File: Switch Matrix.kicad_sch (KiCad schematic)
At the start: 131 parts, among them SW1 SD_6B1D, SW10 SD_4B1E, SW100 SD_4B3E, SW101 SD_4B3E, SW102 SD_4B3E, SW103 SD_4B3E, SW104 SD_4B3E, SW105 SD_4B3E, SW106 SD_4B3E, SW107 SD_4B3E, SW108 SD_4B3E, SW109 SD_4B3E, SW11 SD_4B1E, SW110 SD_4B3E, SW111 SD_4B3E, SW112 SD_6B1D, SW113 SD_4B3E, SW114 SD_4B3E, SW115 UNPOPULATED, SW116 SD_4B3E, SW117 SD_5B3E, SW118 SD_4B3E, SW119 UNPOPULATED, SW12 SD_6B1D, SW120 SD_4B3E, SW121 SD_4B3E, SW122 SD_4B3E, SW122a0 UNPOPULATED, SW123 SD_4B3E, SW123a0 UNPOPULATED, SW124 UNPOPULATED, SW124a0 SD_4B3E, SW125 SD_4B3E, SW126 SD_4B3E, SW127 UNPOPULATED, SW128 SD_4B3E, SW13 SD_4B1E, SW14 SD_6B1D, SW15 SD_4B1E, SW16 SD_6B1D, SW17 SD_4B1E, SW18 SD_6B1D, SW19 SD_4B1E, SW2 SD_4B1E, SW20 SD_6B1D, SW21 SD_4B1E, SW22 SD_6B1D, SW23 SD_4B1E, SW24 SD_6B1D, SW25 SD_4B3E, SW26 SD_4B3E, SW27 SD_6B1D, SW28 SD_4B3E, SW29 SD_4B3E, SW3 SD_6B1D, SW30 SD_4B3E, SW31 SD_4B3E, SW32 SD_4B3E, SW33 SD_4B3E, SW34 SD_4B3E, SW35 SD_4B3E, SW36 SD_4B3E, SW37 SD_4B3E, SW38 SD_4B3E, SW39 SD_4B3E, SW4 SD_4B1E, SW40 SD_4B3E, SW41 UNPOPULATED, SW42 SD_4B3E, SW43 SD_4B3E, SW44 SD_4B3E, SW45 SD_4B3E, SW46 SD_6B1D, SW47 SD_4B3E, SW48 SD_4B3E, SW49 SD_4B3E, SW5 SD_6B1D, SW50 SD_4B3E, SW51 SD_4B3E, SW52 SD_6B1D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

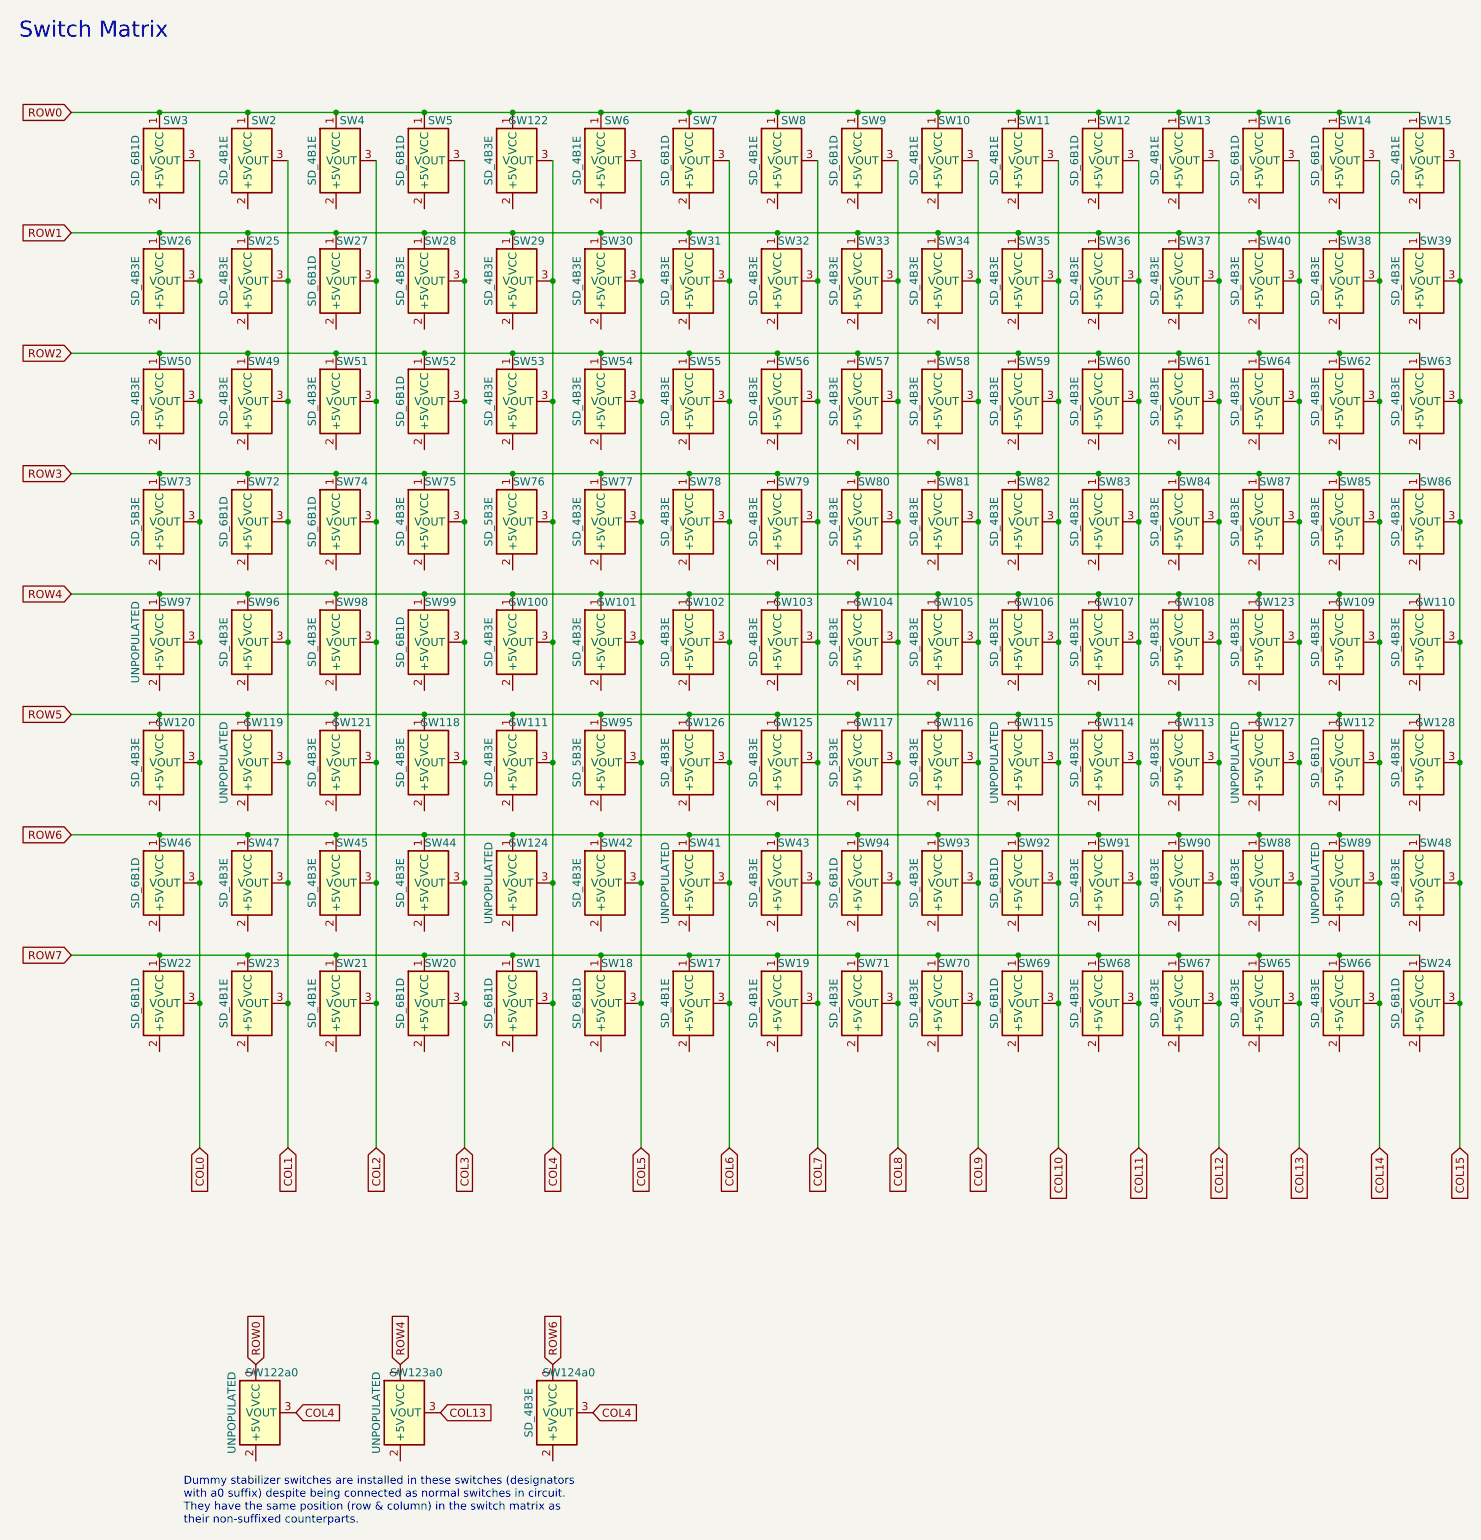
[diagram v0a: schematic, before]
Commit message: wip: footprint and symbols update 1
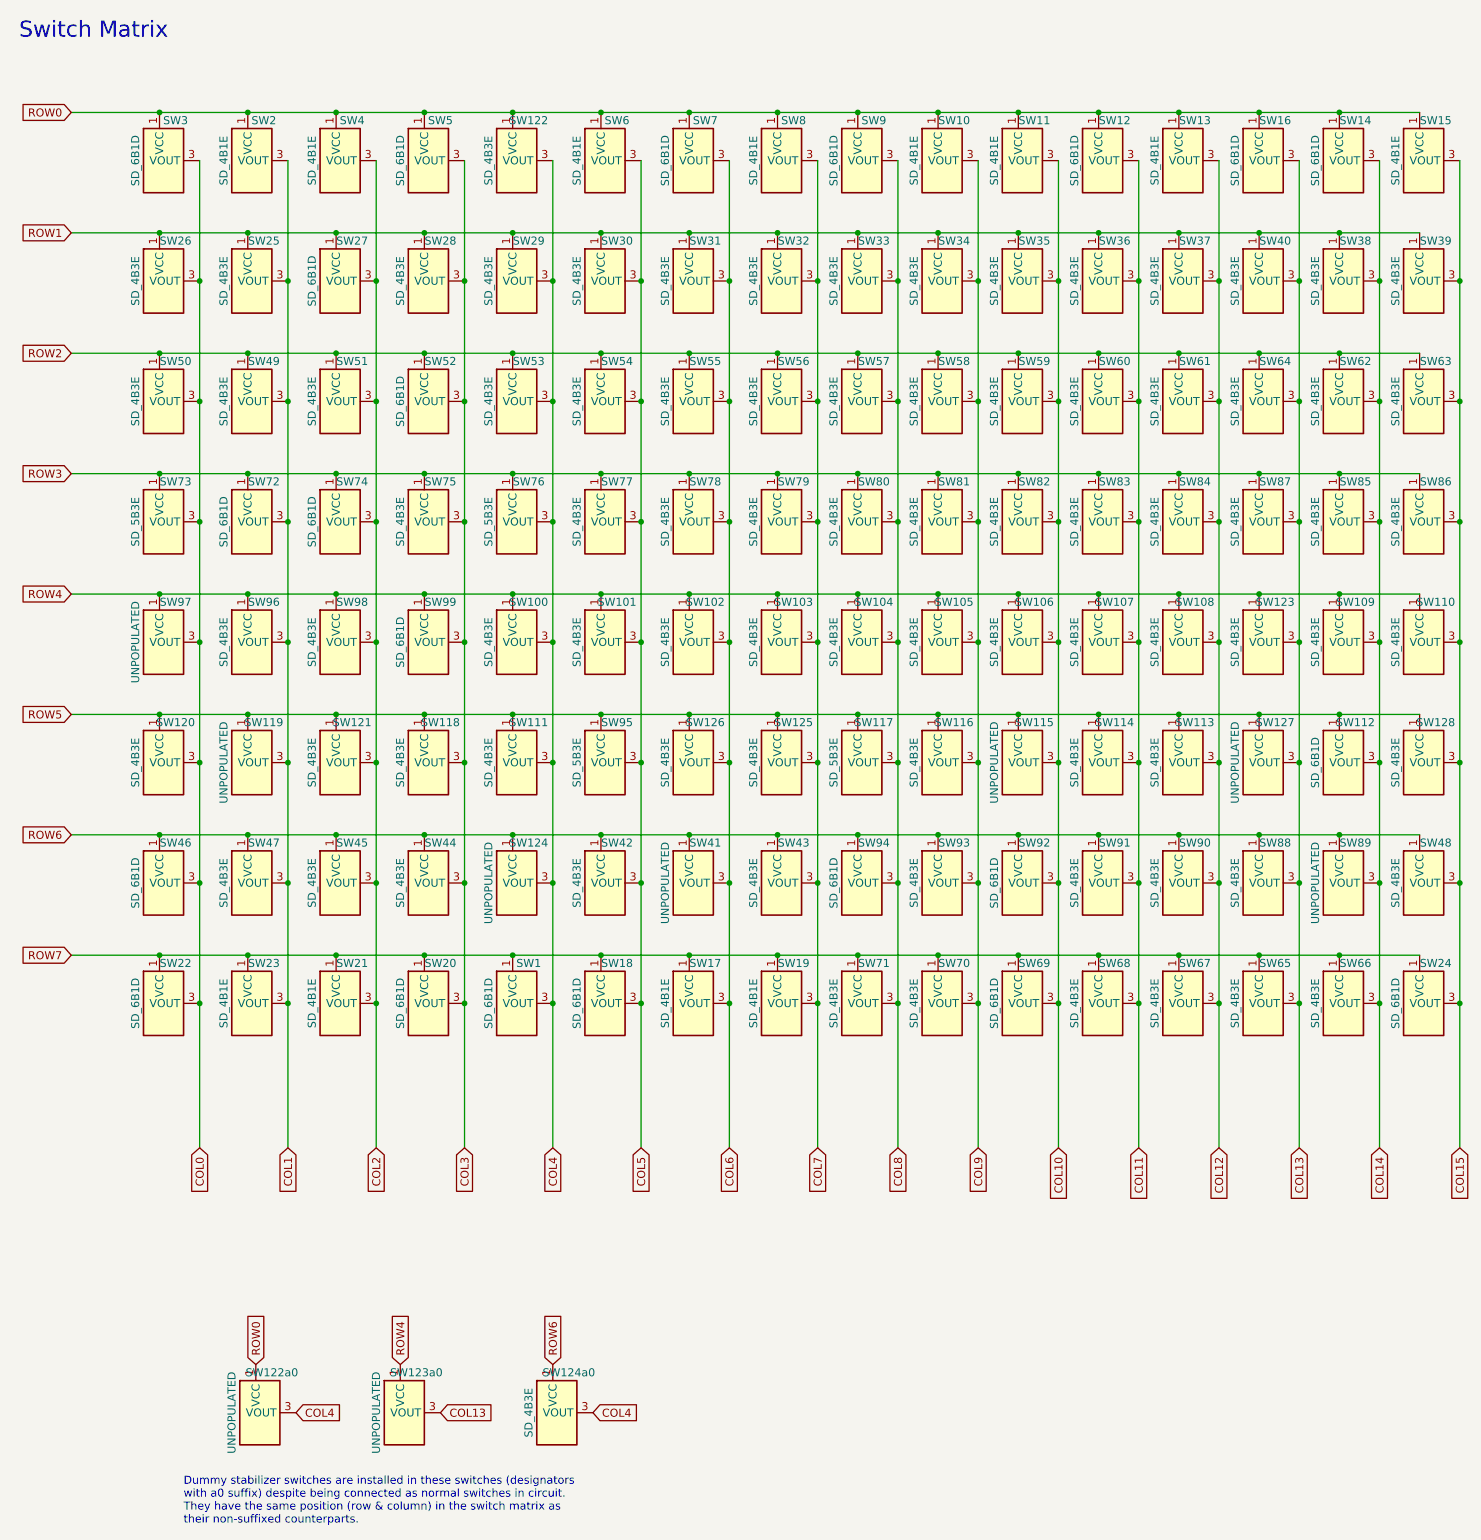
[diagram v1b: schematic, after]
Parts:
- SW1, SW10, SW100, SW101, SW102, SW103, SW104, SW105, SW106, SW107, SW108, SW109, SW11, SW110, SW111, SW112, SW113, SW114, SW115, SW116, SW117, SW118, SW119, SW12, SW120, SW121, SW122, SW122a0, SW123, SW123a0, SW124, SW124a0, SW125, SW126, SW127, SW128, SW13, SW14, SW15, SW16, SW17, SW18, SW19, SW2, SW20, SW21, SW22, SW23, SW24, SW25, SW26, SW27, SW28, SW29, SW3, SW30, SW31, SW32, SW33, SW34, SW35, SW36, SW37, SW38, SW39, SW4, SW40, SW41, SW42, SW43, SW44, SW45, SW46, SW47, SW48, SW49, SW5, SW50, SW51, SW52, SW53, SW54, SW55, SW56, SW57, SW58, SW59, SW6, SW60, SW61, SW62, SW63, SW64, SW65, SW66, SW67, SW68, SW69, SW7, SW70, SW71, SW72, SW73, SW74, SW75, SW76, SW77, SW78, SW79, SW8, SW80, SW81, SW82, SW83, SW84, SW85, SW86, SW87, SW88, SW89, SW9, SW90, SW91, SW92, SW93, SW94, SW95, SW96, SW97, SW98, SW99: symbol MicroSwitch_SD_4B3E:SD_4B3E -> MicroSwitch:MicroSwitchSDSeriesE
